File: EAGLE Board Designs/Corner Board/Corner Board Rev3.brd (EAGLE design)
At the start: 66.5 x 44.9 mm, 40 parts, among them J1 CONNECTOR-8_AMPHENOL_M12A_08P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, J2 CONNECTOR-2_MICROFIT_SMD_RIGH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, J3 CONNECTOR-4_AMPHENOL_M12A_04P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, J4 CONNECTOR-4_μF_S_RA_, J5 CONNECTOR-4_μF_S_RA_, U1 VOLTAGE_REGULATOR_SOT-89_15V, U2 OPAMP_1_CHANNEL_OPA991, U3 INA823DT, U4 OPAMP_1_CHANNEL_OPA991, U5 OPAMP_1_CHANNEL_OPA991, U6 VOLTAGE_REFERENCE_SOIC-8_10V

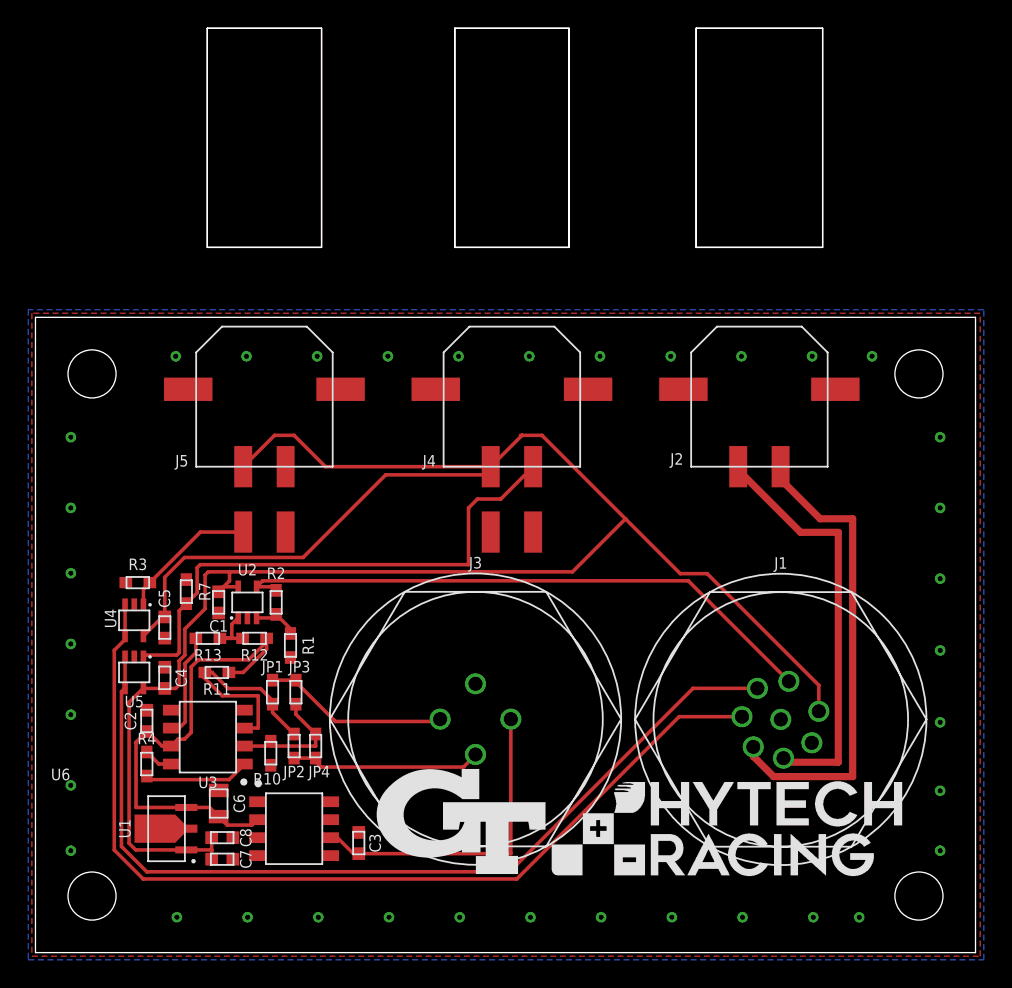
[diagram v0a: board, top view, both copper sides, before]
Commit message: Finalized Corner Board Rev3
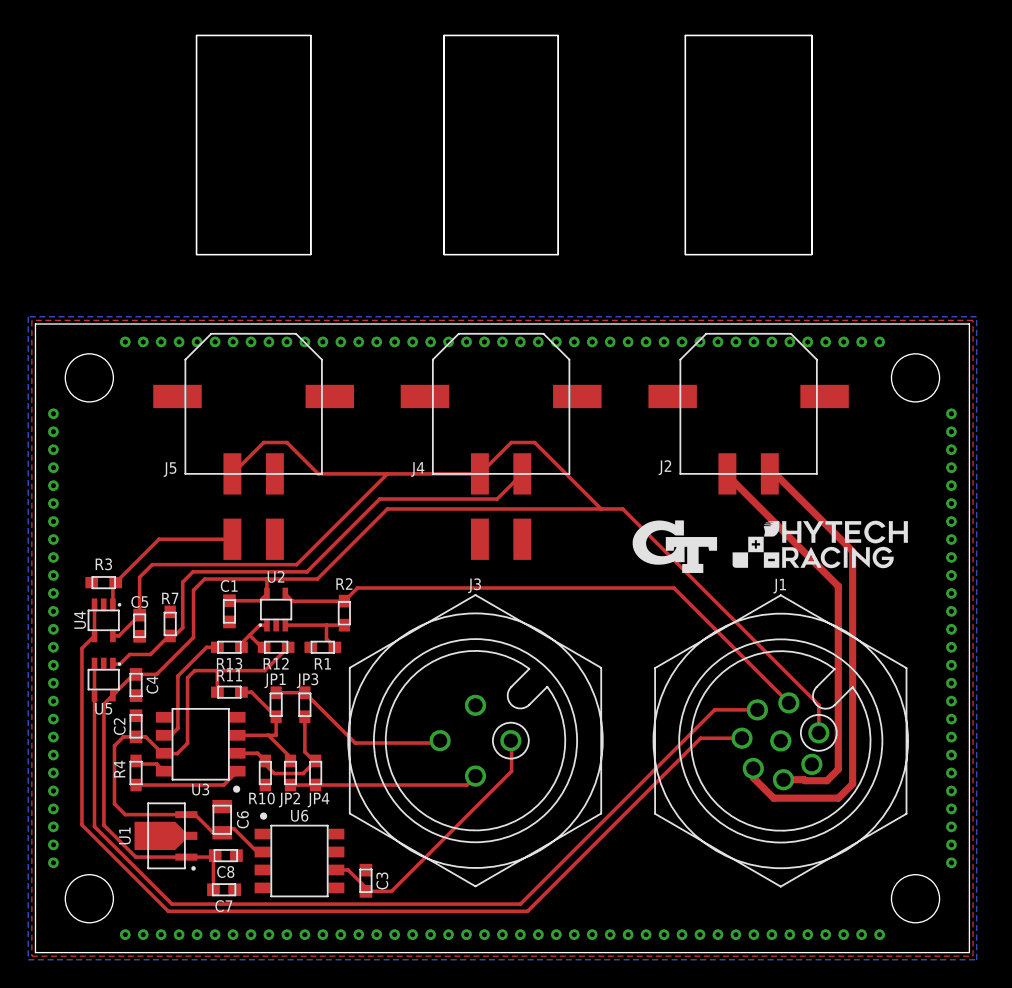
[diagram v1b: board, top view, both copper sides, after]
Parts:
- removed U$13: (no value), HyTechManufacturing:LOGO_HYTECH_MEDIUM
- added U$19: (no value), HyTechManufacturing:LOGO_HYTECH_SMALL
- U$14: device HyTechManufacturing:LOGO_GT_MEDIUM -> HyTechManufacturing:LOGO_GT_SMALL
- moved U$14 24.6 mm to (45.2, 28.7)
- moved R2 4.89 mm to (21.8, 24.0)
- moved C3 2.71 mm to (23.4, 5.08)
- moved R7 2.56 mm to (9.53, 23.2)
- moved R3 2.41 mm to (4.83, 26.2)
- moved U6 2.32 mm to (18.7, 6.48)
- moved R1 2.29 mm to (20.3, 21.6), turned to 0 degrees
- moved U5 2.22 mm to (4.83, 19.3)
- moved C7 2.16 mm to (13.3, 4.45)
- moved U4 2.16 mm to (4.83, 23.5)
- moved C4 2.09 mm to (7.11, 18.9), turned to 270 degrees
- moved U2 2.09 mm to (17.0, 24.3)
- moved JP2 1.92 mm to (18.0, 12.7)
- moved JP4 1.91 mm to (19.8, 12.7)
- moved C5 1.78 mm to (7.37, 23.1)
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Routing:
- net N$9: track 16.8 -> 9.68 mm
- net 10V: track 22.7 -> 18.9 mm
- net N$1: track 3.25 -> 5.99 mm
- net LOAD_CELL_AMPLIFIED: track 42.2 -> 39.6 mm
- net 15V: track 34.1 -> 36.8 mm
- net SUS_POT_2_24V: track 67.6 -> 70.2 mm
- net SUS_POT_1_24V: track 64.6 -> 66.3 mm
- net SUS_POT_1: track 38.2 -> 36.6 mm
- net N$7: track 9.04 -> 10.5 mm
- net SUS_POT_2: track 9.84 -> 11.2 mm
- net +24V: track 147.7 -> 146.4 mm
- net N$3: track 7.77 -> 8.53 mm
- net POSTINTERLOCK: track 29.4 -> 28.8 mm
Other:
- board size 66.5 x 44.9 mm -> 66 x 44.5 mm
